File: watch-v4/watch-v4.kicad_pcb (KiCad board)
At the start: 4 copper layers, 35 x 35 mm, 38 parts, among them J1 CONN_10, Q1 MOSFET_P, SW1 SPST, SW2 SPST, SW3 SPST, U1 IC_MCP73831, U2 MAX1722, U3 DS3231, U4 LSM9DS0, U5 NRF51822, U6 BALUN, U7 NeoPixel, X1 16mhz

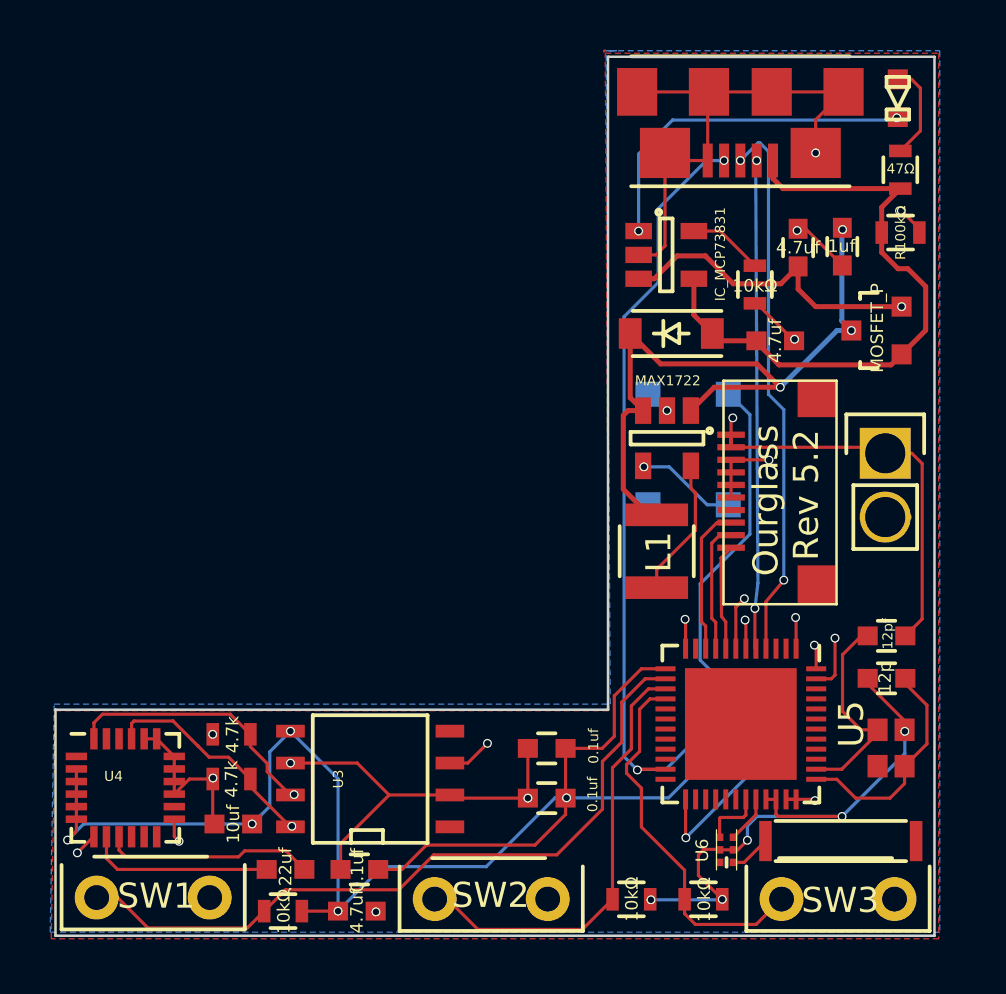
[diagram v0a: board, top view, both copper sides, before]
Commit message: further v6 work; incomplete
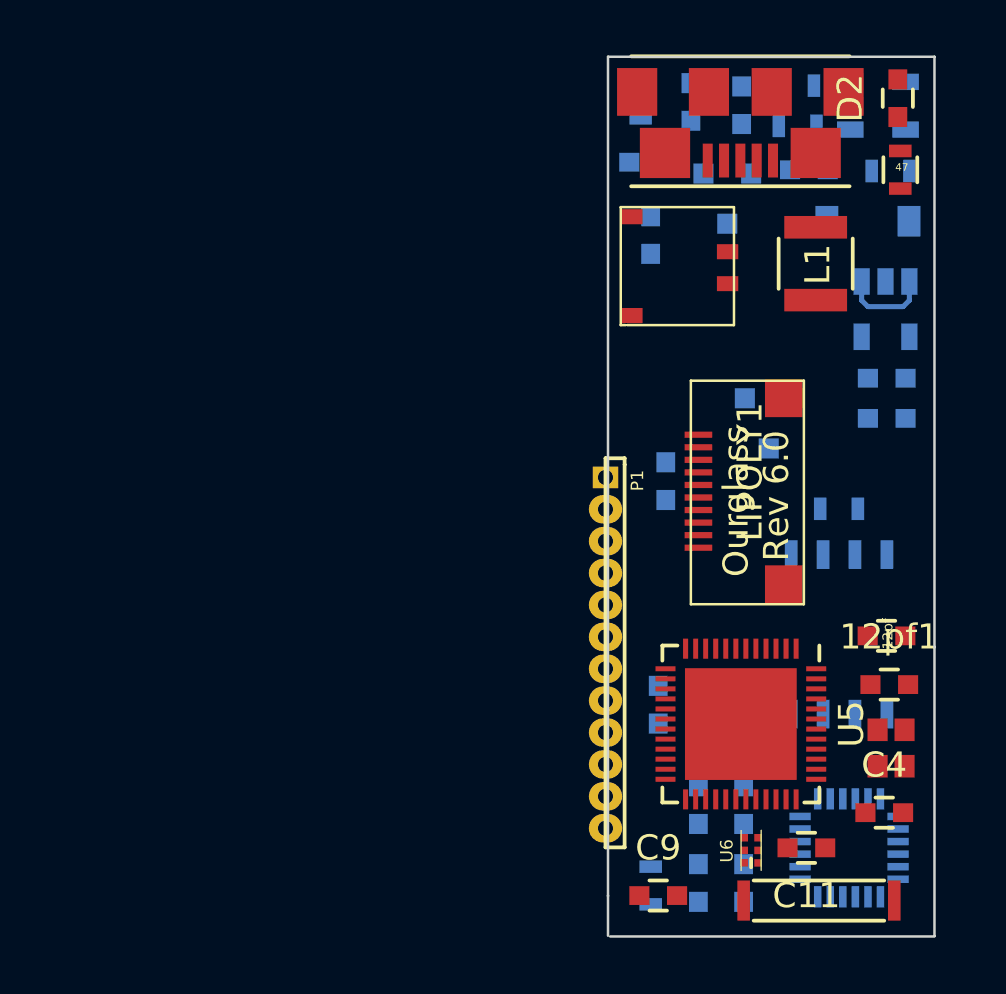
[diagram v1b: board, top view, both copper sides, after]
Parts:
- removed 12p: C9, Capacitors_SMD:C_0603
- removed SW1, SW2, SW3: SPST, watch-v4:SW_Tactile_SPST_Angled_no_anchors
- removed U7: NeoPixel, LEDs:Neopixel
- added 12pf1: C9, Capacitors_SMD:C_0603, F.Cu at (183.4, 105.7)
- added C11: 2n2, Capacitors_SMD:C_0603, F.Cu at (180.1, 112.2)
- added C12: 1u, Capacitors_SMD:C_0603, B.Cu at (180.2, 85.2)
- added C4: 100n, Capacitors_SMD:C_0603, F.Cu at (183.2, 110.8)
- added C9: 47n, Capacitors_SMD:C_0603, F.Cu at (174.2, 114.1)
- added D3: LED, Capacitors_SMD:C_0603, B.Cu at (174.2, 106.5)
- added D4: LED, Capacitors_SMD:C_0603, B.Cu at (174.5, 97.6)
- added D5: LED, Capacitors_SMD:C_0603, B.Cu at (173.9, 87.8)
- added P1: Expansion Header, Socket_Strips:Socket_Strip_Straight_1x12_small, F.Cu at (172.1, 103.8)
- added Q2: BSS138, TO_SOT_Packages_SMD:SOT-23, B.Cu at (178.6, 95.3)
- added R9: 47, Resistors_SMD:R_0603, B.Cu at (173.9, 113.7)
- C1, C2, C5, C6, C7, C8, D1, Q1, R5, R6, U1, U2, U3, U4: moved to B.Cu
- C13: value 0.1uf -> 0u1; moved to B.Cu
- C14: value 0.1uf -> 1nf; moved to B.Cu
- C3: value 4.7uf -> 4u7; moved to B.Cu
- D2: footprint LED-0603 -> Capacitors_SMD:C_0603
- LIPOLY1: footprint watch-v4:Pin_Header_Straight_1x02 -> Socket_Strips:molex_2_pos
- R1: value 47Ω -> 47
- R2, R4: value 10kΩ -> 10k; moved to B.Cu
- R3: value R100kΩ -> 100k; moved to B.Cu
- R7, R8: value 10kΩ -> 10M; moved to B.Cu
- moved R7 33.0 mm to (179.7, 81.8)
- moved R8 31.0 mm to (179.8, 83.5)
- moved U4 28.9 mm to (181.8, 112.2), turned to 90 degrees
- moved R4 27.3 mm to (181.4, 98.7)
- moved C14 21.5 mm to (183.3, 93.5), turned to 0 degrees
- moved R5 20.6 mm to (177.8, 107.6), turned to 270 degrees
- moved U3 19.5 mm to (181.4, 103.7), turned to 0 degrees
- moved R6 18.9 mm to (176.0, 107.5), turned to 270 degrees
- moved C13 18.9 mm to (183.3, 95.1), turned to 0 degrees
- moved C7 18.5 mm to (175.8, 110.5), turned to 90 degrees
- moved C5 16.4 mm to (175.8, 113.6), turned to 270 degrees
- moved C8 15.5 mm to (177.6, 110.5), turned to 90 degrees
- moved C6 15.4 mm to (177.6, 113.6), turned to 270 degrees
- moved L1 13.1 mm to (180.5, 88.9)
- moved R3 11.6 mm to (173.5, 82.4), turned to 90 degrees
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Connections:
- net DISPLAY_MOSI renamed /Display_MOSI
- net DISPLAY_SCK renamed /Display_SCK
- net DISPLAY_SS renamed /Display_SS
- net Net-(12pf1-Pad2) renamed /XC2
- net Net-(C10-Pad1) renamed /XC1
- net Net-(U5-Pad31) renamed /Bal1
- net Net-(U5-Pad32) renamed /Bal2
- C13 pad 2: VCC -> /VCC
- C14 pad 2: VCC -> /VCC
- C7 pad 1: VCC -> /VCC
- C8 pad 1: VCC -> /VCC
- J1 pad 5: VCC -> /VCC
- J1 pad 6: VCC -> /VCC
- J1 pad 7: VCC -> /VCC
- J1 pad 8: VCC -> /VCC
- R4 pad 1: /SW1 -> /VCC
- R4 pad 2: GND -> /ClockINT
- R5 pad 1: SDA -> /SCL
- R5 pad 2: VCC -> /VCC
- R6 pad 1: SCL -> /SDA
- R6 pad 2: VCC -> /VCC
- R7 pad 1: /SW2 -> /VBAT
- R7 pad 2: GND -> /BatterySense
- R8 pad 1: GND -> /BatterySense
- R8 pad 2: /SW3 -> GND
- U2 pad 4: VCC -> /VCC
- U3 pad 2: VCC -> /VCC
- U3 pad 6: VCC -> /VCC
- U3 pad 7: SDA -> /SCL
- U3 pad 8: SCL -> /SDA
- U4 pad 15: VCC -> /VCC
- U4 pad 16: VCC -> /VCC
- U4 pad 17: VCC -> /VCC
- U4 pad 18: VCC -> /VCC
- U4 pad 19: VCC -> /VCC
- U4 pad 20: VCC -> /VCC
- U4 pad 21: SCL -> /SCL
- U4 pad 24: SDA -> /SDA
- U5 pad 1: VCC -> /VCC
- U5 pad 12: VCC -> /VCC
- U5 pad 14: /SW1 -> /EX8
- U5 pad 15: /SW2 -> /EX9
- U5 pad 16: /SW3 -> /EX10
- U5 pad 17: Net-(U5-Pad17) -> /EX11
- U5 pad 18: Net-(U5-Pad18) -> /EX12
- U5 pad 19: Net-(U5-Pad19) -> /EX13
- U5 pad 20: Net-(U5-Pad20) -> /EX14
- U5 pad 21: Net-(U5-Pad21) -> /EX15
- U5 pad 22: Net-(U5-Pad22) -> /BatterySense
- U5 pad 30: Net-(U5-Pad30) -> /VDD_PA
- U5 pad 35: VCC -> /VCC
- U5 pad 36: VCC -> /VCC
- U5 pad 6: SCL -> /SCL
- U5 pad 7: SDA -> /SDA
- U6 pad 5: GND -> /VDD_PA
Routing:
- net GND: track 148.3 -> 0.00 mm, vias 16 -> 0
- net VCC: track 92.6 -> 0.00 mm, vias 9 -> 0
- net SDA: track 33.9 -> 0.00 mm, vias 2 -> 0
- net /Reset: track 32.1 -> 0.00 mm, vias 2 -> 0
- net SCL: track 31.6 -> 0.00 mm, vias 2 -> 0
- net /Accel_INT: track 30.6 -> 0.00 mm, vias 2 -> 0
- net /SW1: track 29.3 -> 0.00 mm
- net /EXTVCC: track 25.0 -> 0.00 mm
- net /Regulator_In: track 28.0 -> 3.61 mm, vias 3 -> 0
- net /VBAT: track 24.0 -> 0.00 mm, vias 1 -> 0
- net /Backlight: track 22.1 -> 0.00 mm, vias 1 -> 0
- net /TX: track 22.0 -> 0.00 mm, vias 2 -> 0
- net /ClockINT: track 21.4 -> 0.00 mm, vias 2 -> 0
- net /RX: track 19.5 -> 0.00 mm, vias 2 -> 0
- net /SW2: track 17.7 -> 0.00 mm
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- removed copper zone on B.Cu, net GND
- removed copper zone on F.Cu, net GND
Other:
- board size 35 x 35 mm -> 13 x 35 mm
- board text added: "Ourglass Rev 6.0"
- board text removed: "Ourglass Rev 5.2"
